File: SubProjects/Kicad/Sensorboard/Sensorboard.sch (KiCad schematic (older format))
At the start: 16 parts, among them P1 ToyRaceCar_V2_REV3_J4, P2 ToyRaceCar_V2_REV3_J3, P3 ToyRaceCar_V2_REV3_J2, P4 ToyRaceCar_V2_REV3_J1, P5 MPU-6050, P6 ToyRaceCar_V2_REV3_J5, P7 CNY70, P8 SS495A, Q1 BSS138, Q2 BSS138

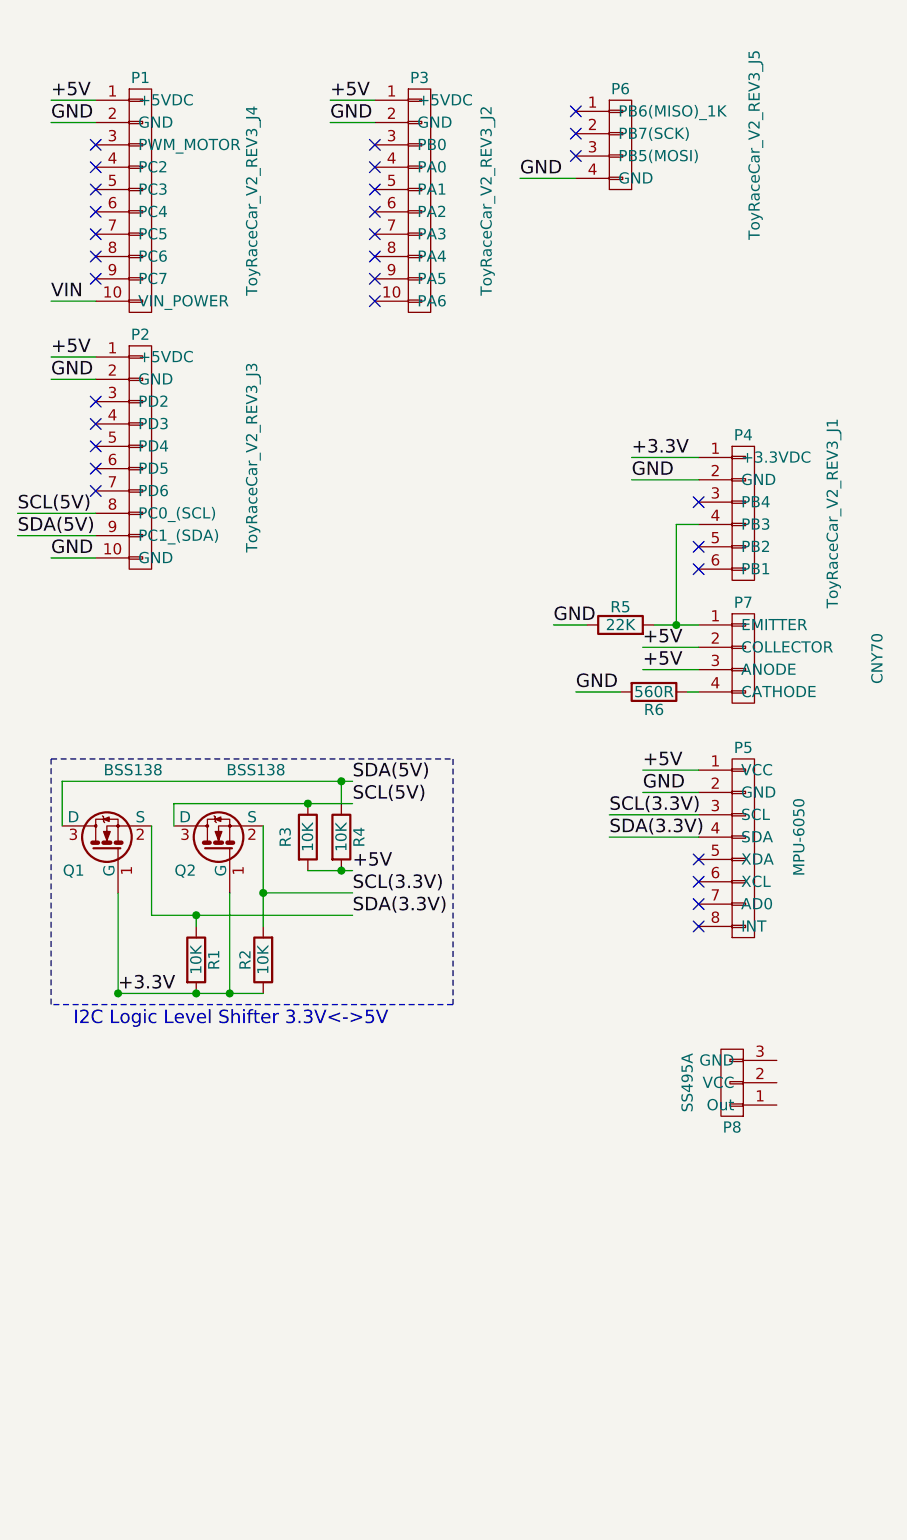
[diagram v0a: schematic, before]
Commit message: Nearly final design. Just missing the mounting holes
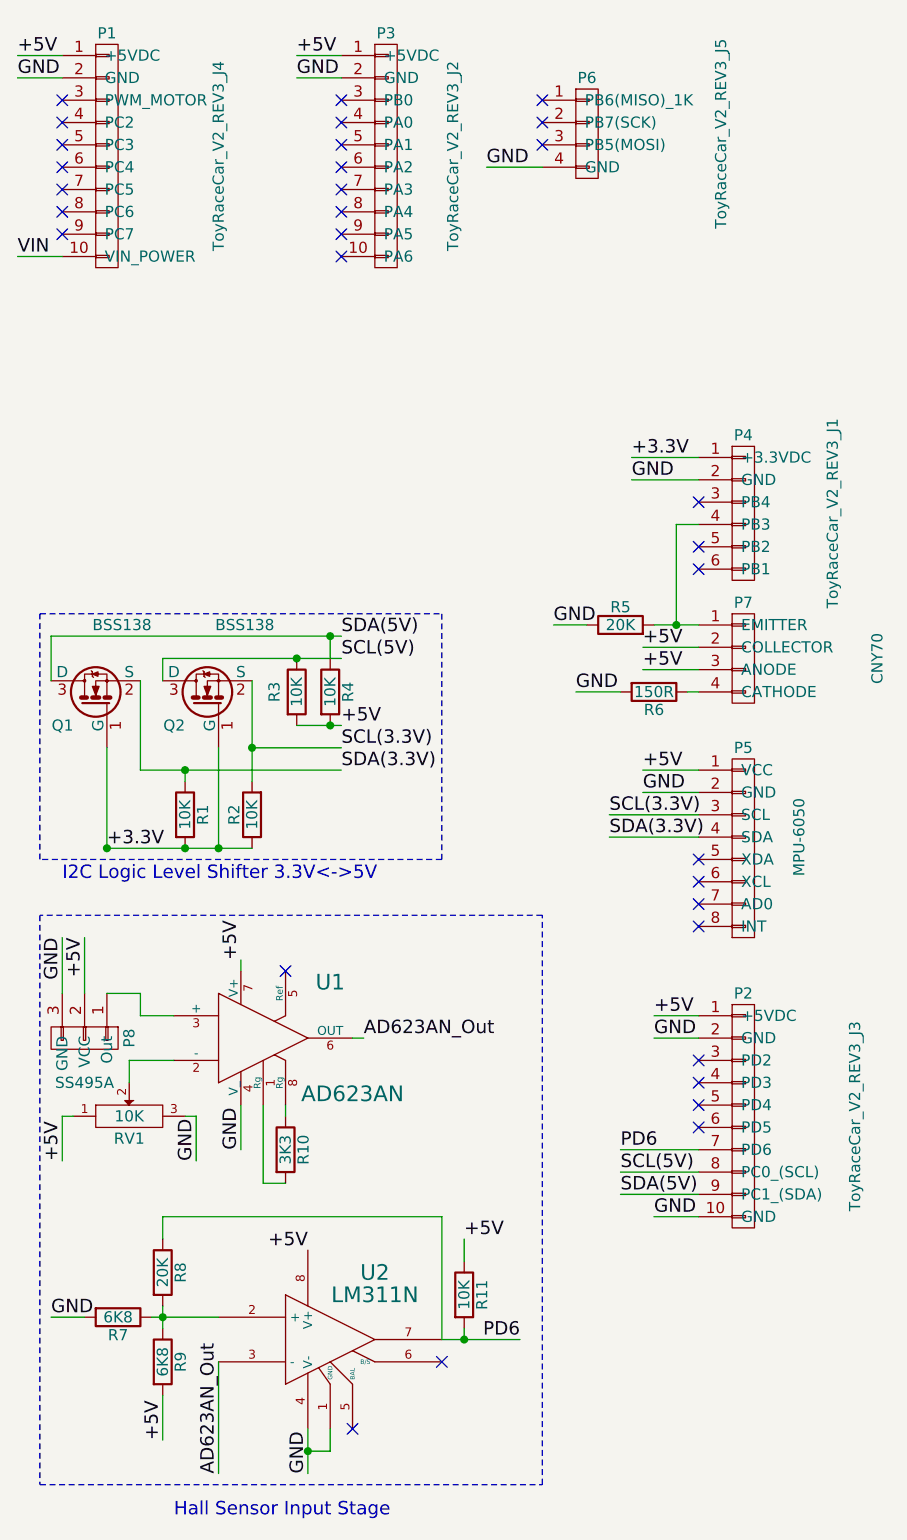
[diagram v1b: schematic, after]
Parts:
- added R10: 3K3, Resistors_SMD:R_0805_HandSoldering, symbol R
- added R11: 10K, Resistors_SMD:R_0805_HandSoldering, symbol R
- added R7, R9: 6K8, Resistors_SMD:R_0805_HandSoldering, symbol R
- added R8: 20K, Resistors_SMD:R_0805_HandSoldering, symbol R
- added RV1: 10K, Potentiometers:Potentiometer_Bourns_3006P_Angular_ScrewFront, symbol POT
- added U1: AD623AN, Housings_DIP:DIP-8__300, symbol AD623AN
- added U2: LM311N, Housings_DIP:DIP-8__300, symbol LM311N
- P8: footprint Sensorboard:KK254-3 -> (none)
- R1, R2, R3, R4: footprint Resistors_SMD:R_0603_HandSoldering -> Resistors_SMD:R_0805_HandSoldering
- R5: value 22K -> 20K; footprint Resistors_SMD:R_0603_HandSoldering -> Resistors_SMD:R_0805_HandSoldering
- R6: value 560R -> 150R; footprint Resistors_SMD:R_0603_HandSoldering -> Resistors_SMD:R_0805_HandSoldering
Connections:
- net +5V: now also P8.2 (VCC), R11.1, R9.2, RV1.1, U1.7 (V+), U2.8 (V+)
- net GND: now also P8.3 (GND), R7.2, RV1.3, U1.4 (V_), U2.1 (GND), U2.4 (V-)
- net PD6: now reaches P2.7 (PD6)
- net PD6: now also R11.2, R8.1, U2.7
- net at P8.1 (Out): now also U1.3 (+)
- new net: R10.2, U1.1 (Rg)
- new net: RV1.2, U1.2 (-)
- new net: R10.1, U1.8 (Rg)
- new net: R7.1, R8.2, R9.1, U2.2 (+)
- new net AD623AN_Out: U1.6 (OUT), U2.3 (-)
- no-connect marks 30 -> 32
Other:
- note added: "Hall Sensor Input Stage"
- moved on the sheet: P1, P2, P3, P6, Q1, Q2, R1, R2, R3, R4
